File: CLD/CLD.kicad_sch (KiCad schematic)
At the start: 30 parts, among them J1 Conn_01x02, J2 Conn_01x02, J3 Conn_01x02, J4 Conn_01x02, J5 Conn_02x05_Counter_Clockwise, Q1 BSC072N08NS5, U1 STM32F103TBUx, U2 FAN3111E, U3 INA180A1, U4 MCP2551-I-SN

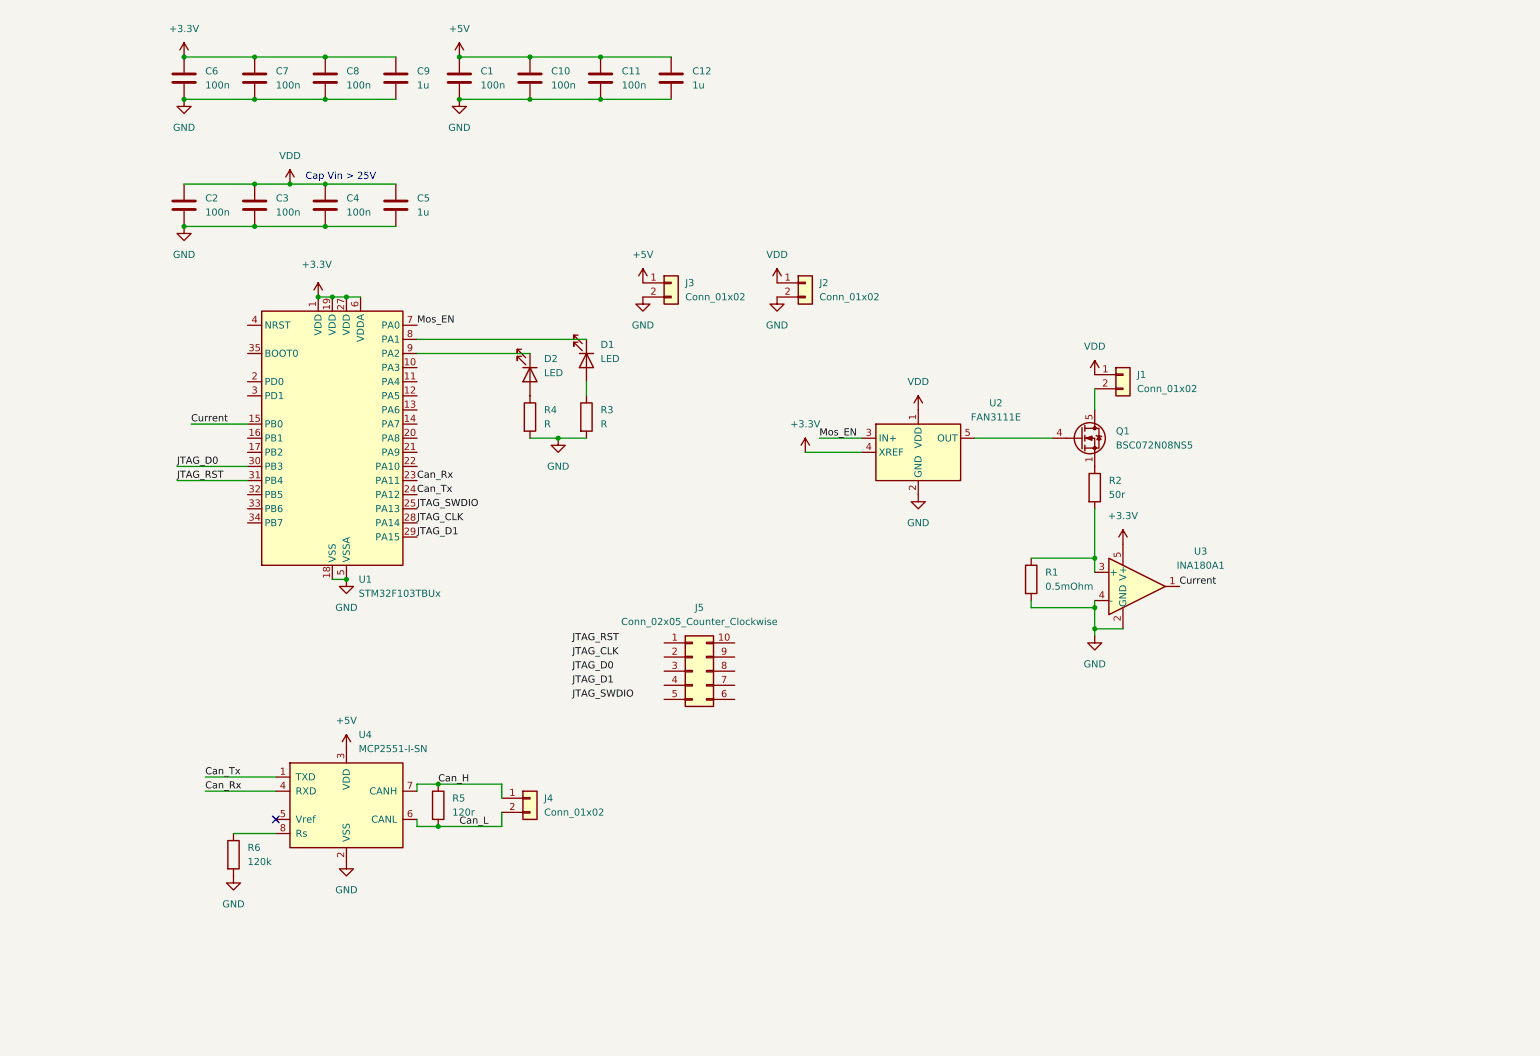
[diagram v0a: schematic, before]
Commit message: update 17/09
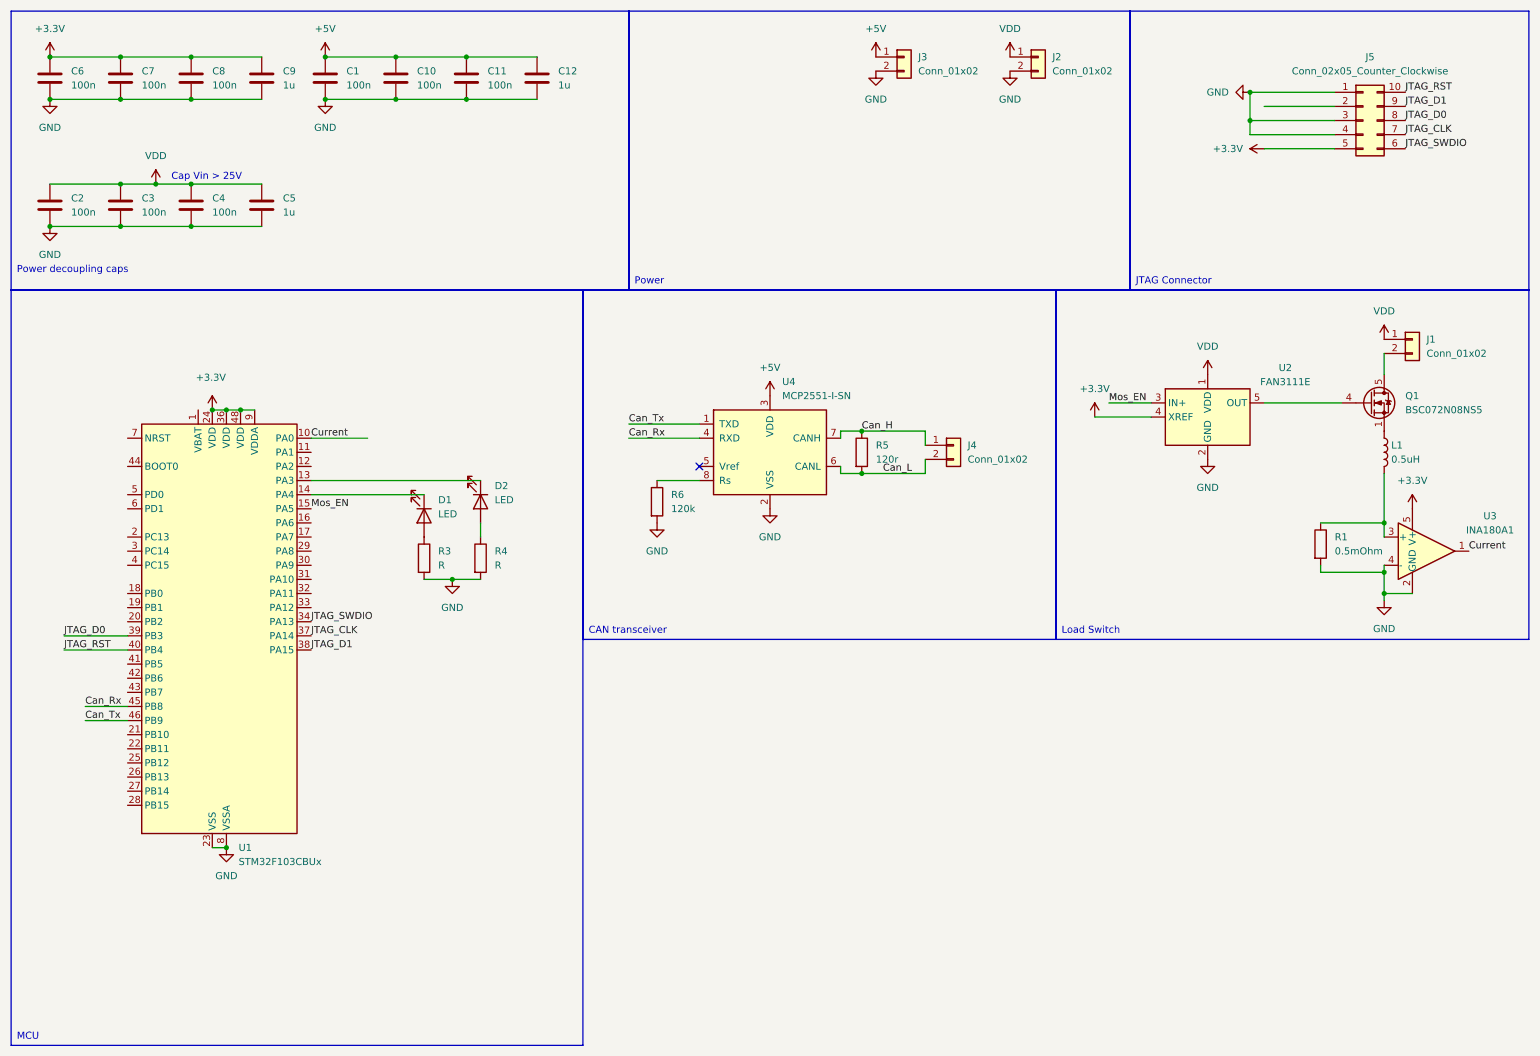
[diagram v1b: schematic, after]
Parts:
- removed R2: 50r, symbol Device:R
- removed U1: STM32F103TBUx, Package_DFN_QFN:QFN-36-1EP_6x6mm_P0.5mm_EP4.1x4.1mm, symbol MCU_ST_STM32F1:STM32F103TBUx
- added L1: 0.5uH, Inductor_SMD:L_Bourns-SRN8040_8x8.15mm, symbol Device:L
- added U1: STM32F103CBUx, Package_DFN_QFN:QFN-48-1EP_7x7mm_P0.5mm_EP5.6x5.6mm, symbol MCU_ST_STM32F1:STM32F103CBUx
- C1, C10, C11, C12, C2, C3, C4, C5, C6, C7, C8, C9: footprint (none) -> Capacitor_SMD:C_0201_0603Metric
- D1, D2: footprint (none) -> Diode_SMD:D_0201_0603Metric
- J1, J2, J3, J4: footprint (none) -> Connector_PinHeader_2.54mm:PinHeader_1x02_P2.54mm_Vertical
- J5: footprint (none) -> Connector_PinHeader_1.27mm:PinHeader_2x05_P1.27mm_Vertical_SMD
- R1: footprint (none) -> Resistor_SMD:R_Shunt_Vishay_WSK2512_6332Metric_T1.19mm
- R3, R4, R5, R6: footprint (none) -> Resistor_SMD:R_0201_0603Metric
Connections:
- net +3.3V: now also J5.5 (Pin_5), U1.24 (VDD), U1.36 (VDD), U1.48 (VDD), U1.9 (VDDA)
- net Can_Rx: now also U1.45 (PB8)
- net Can_Tx: now also U1.46 (PB9)
- net Current: now also U1.10 (PA0)
- net GND: now also J5.1 (Pin_1), J5.3 (Pin_3), J5.4 (Pin_4), U1.23 (VSS), U1.35 (VSS), U1.47 (VSS), U1.49 (VSS), U1.8 (VSSA)
- net JTAG_CLK: now also J5.7 (Pin_7), U1.37 (PA14)
- net JTAG_D0: now also J5.8 (Pin_8), U1.39 (PB3)
- net JTAG_D1: now also J5.9 (Pin_9), U1.38 (PA15)
- net JTAG_RST: now also J5.10 (Pin_10), U1.40 (PB4)
- net JTAG_SWDIO: now also J5.6 (Pin_6), U1.34 (PA13)
- net Mos_EN: now also U1.15 (PA5)
- net at Q1.1 (S), Q1.2 (S), Q1.3 (S): now also L1.1
- net at R1.1, U3.3 (+): now also L1.2
- net at D2.1 (K): now also U1.13 (PA3)
- net at D1.1 (K): now also U1.14 (PA4)
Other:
- moved on the sheet: C1, C10, C11, C12, C2, C3, C4, C5, C6, C7, C8, C9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
